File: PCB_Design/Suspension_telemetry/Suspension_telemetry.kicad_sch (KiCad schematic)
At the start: 23 parts, among them J11 530480310, J12 530480410, J2 Conn_01x03_Pin, J3 112J-TDAR-R01, J4 Conn_02x04_Top_Bottom, J6 Conn_01x08_Socket, J7 530480510, J8 530480310, J9 530480410, U5 USBLC6-2SC6

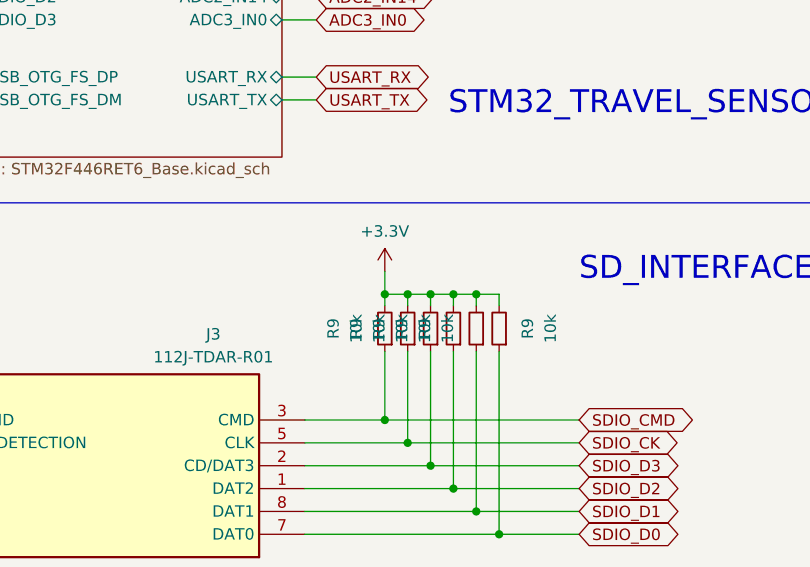
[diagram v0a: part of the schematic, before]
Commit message: Initial:GUI
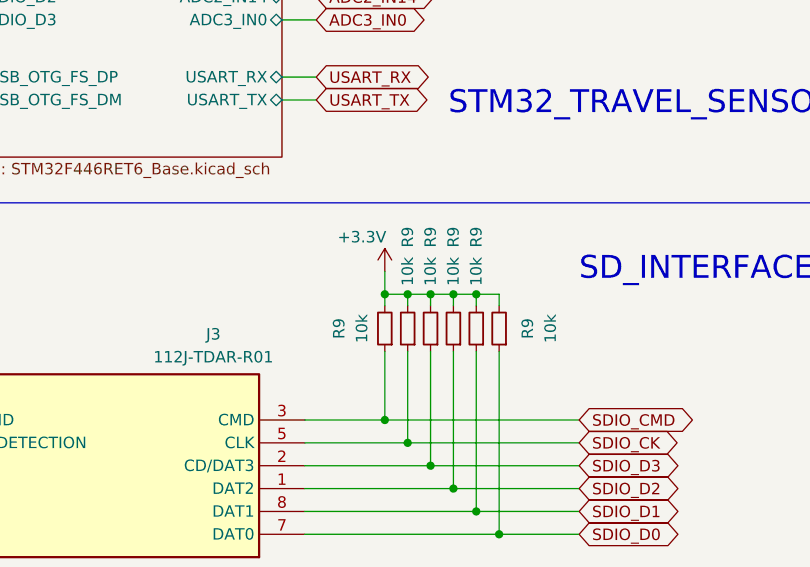
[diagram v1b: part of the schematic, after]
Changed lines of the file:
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@@
   )
   (symbol (lib_id "Device:R_Small") (at 92.71 77.47 180) (unit 1)
-    (in_bom yes) (on_board yes) (dnp no) (fields_autoplaced)
-    (property "Reference" "R9" (at 86.995 77.47 90)
-      (effects (font (size 1.27 1.27)))
-    )
-    (property "Value" "10k" (at 89.535 77.47 90)
+    (in_bom yes) (on_board yes) (dnp no)
+    (property "Reference" "R9" (at 92.71 67.31 90)
+      (effects (font (size 1.27 1.27)))
+    )
+    (property "Value" "10k" (at 92.71 71.12 90)
       (effects (font (size 1.27 1.27)))
     )
@@
   )
   (symbol (lib_id "Device:R_Small") (at 90.17 77.47 180) (unit 1)
-    (in_bom yes) (on_board yes) (dnp no) (fields_autoplaced)
-    (property "Reference" "R9" (at 84.455 77.47 90)
-      (effects (font (size 1.27 1.27)))
-    )
-    (property "Value" "10k" (at 86.995 77.47 90)
+    (in_bom yes) (on_board yes) (dnp no)
+    (property "Reference" "R9" (at 90.17 67.31 90)
+      (effects (font (size 1.27 1.27)))
+    )
+    (property "Value" "10k" (at 90.17 71.12 90)
       (effects (font (size 1.27 1.27)))
     )
@@
   )
   (symbol (lib_id "power:+3.3V") (at 87.63 71.12 0) (unit 1)
-    (in_bom yes) (on_board yes) (dnp no) (fields_autoplaced)
+    (in_bom yes) (on_board yes) (dnp no)
     (property "Reference" "#PWR024" (at 87.63 74.93 0)
       (effects (font (size 1.27 1.27)) hide)
     )
-    (property "Value" "+3.3V" (at 87.63 66.675 0)
+    (property "Value" "+3.3V" (at 85.09 67.31 0)
       (effects (font (size 1.27 1.27)))
     )
@@
   )
   (symbol (lib_id "Device:R_Small") (at 95.25 77.47 180) (unit 1)
-    (in_bom yes) (on_board yes) (dnp no) (fields_autoplaced)
-    (property "Reference" "R9" (at 89.535 77.47 90)
-      (effects (font (size 1.27 1.27)))
-    )
-    (property "Value" "10k" (at 92.075 77.47 90)
+    (in_bom yes) (on_board yes) (dnp no)
+    (property "Reference" "R9" (at 95.25 67.31 90)
+      (effects (font (size 1.27 1.27)))
+    )
+    (property "Value" "10k" (at 95.25 71.12 90)
       (effects (font (size 1.27 1.27)))
     )
@@
   )
   (symbol (lib_id "Device:R_Small") (at 87.63 77.47 180) (unit 1)
-    (in_bom yes) (on_board yes) (dnp no) (fields_autoplaced)
-    (property "Reference" "R9" (at 81.915 77.47 90)
-      (effects (font (size 1.27 1.27)))
-    )
-    (property "Value" "10k" (at 84.455 77.47 90)
+    (in_bom yes) (on_board yes) (dnp no)
+    (property "Reference" "R9" (at 82.55 77.47 90)
+      (effects (font (size 1.27 1.27)))
+    )
+    (property "Value" "10k" (at 85.09 77.47 90)
       (effects (font (size 1.27 1.27)))
     )
@@
   )
   (symbol (lib_id "Device:R_Small") (at 97.79 77.47 180) (unit 1)
-    (in_bom yes) (on_board yes) (dnp no) (fields_autoplaced)
-    (property "Reference" "R9" (at 92.075 77.47 90)
-      (effects (font (size 1.27 1.27)))
-    )
-    (property "Value" "10k" (at 94.615 77.47 90)
-      (effects (font (size 1.27 1.27)))
-    )
+    (in_bom yes) (on_board yes) (dnp no)
+    (property "Reference" "R9" (at 97.79 67.31 90)
+      (effects (font (size 1.27 1.27)))
+    )
+    (property "Value" "10k" (at 97.79 71.12 90)
+      (effects (font (size 1.27 1.27)))
+    )
